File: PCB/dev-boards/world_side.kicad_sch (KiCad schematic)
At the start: 1 part, among them U1 NUCLEO-F429ZI

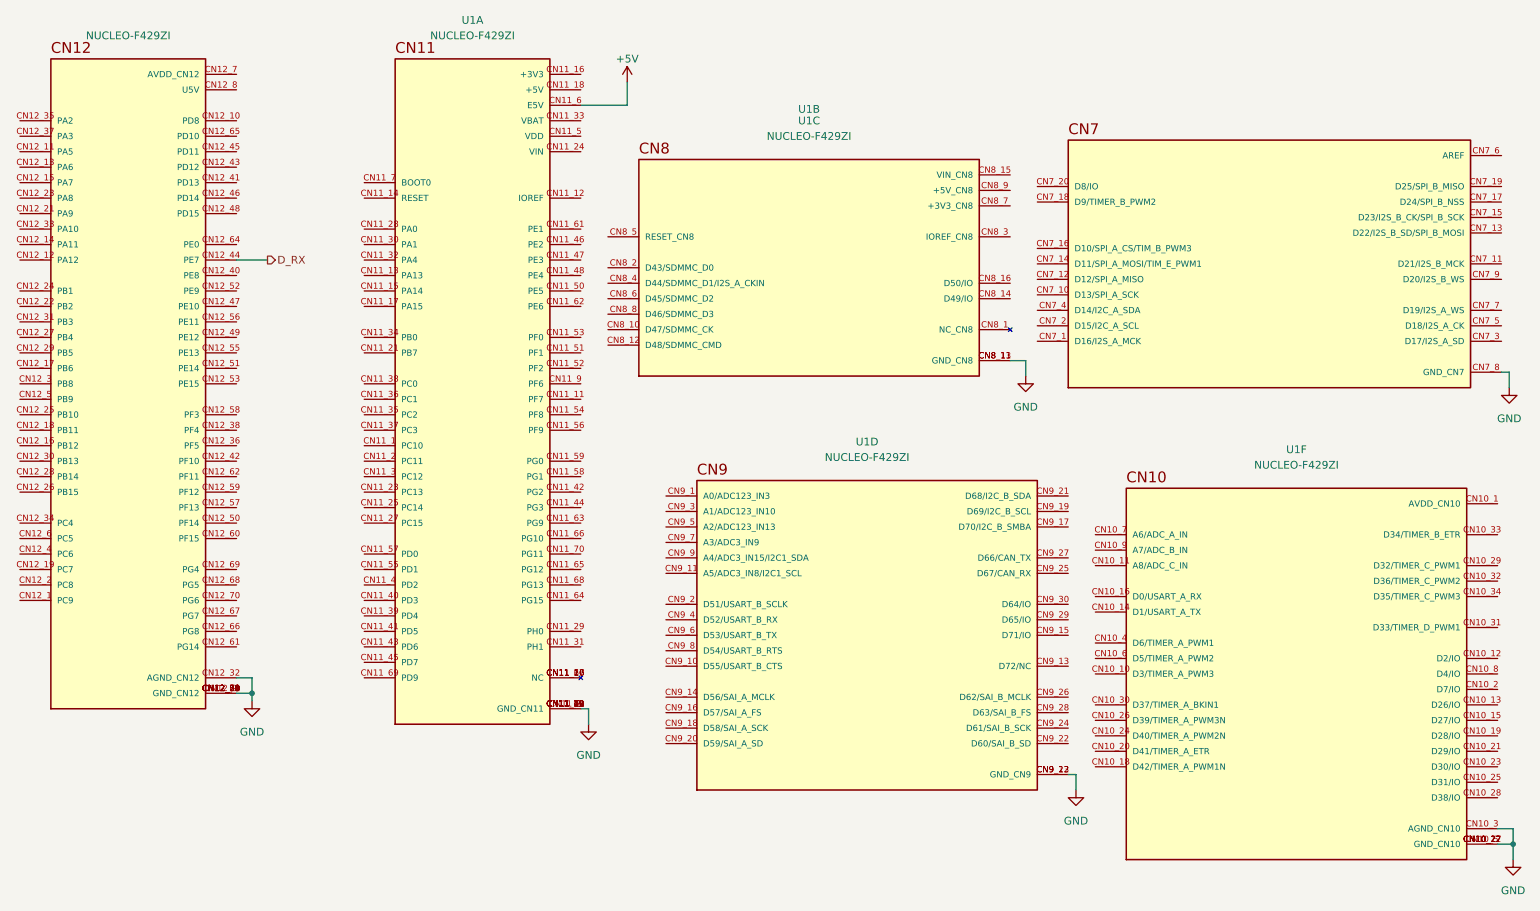
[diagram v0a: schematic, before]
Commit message: PCB board updates
Signed-off-by: Andrew Balmos <abalmos@purdue.edu>
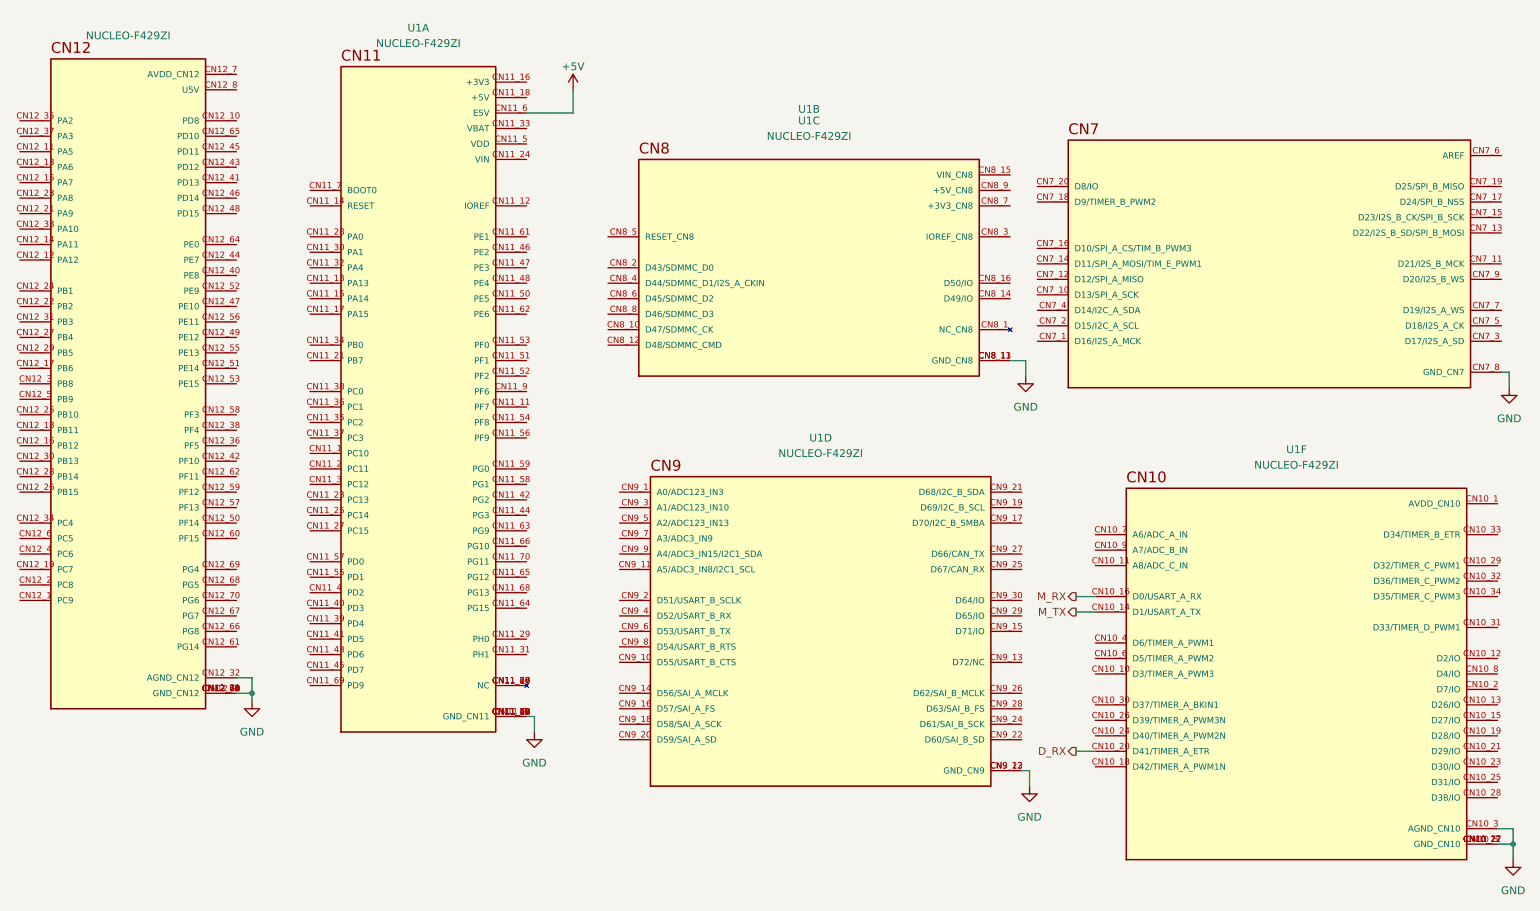
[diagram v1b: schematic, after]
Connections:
- net D_RX: now also U1.CN10_20 (D41/TIMER_A_ETR); no longer U1.CN12_44 (PE7)
- net M_TX: now reaches U1.CN10_14 (D1/USART_A_TX)
- net M_RX: now reaches U1.CN10_16 (D0/USART_A_RX)
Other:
- moved on the sheet: U1A, U1D
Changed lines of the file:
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@@
   (junction (at 55.245 128.27) (diameter 0) (color 0 0 0 0)
   )
-  (wire (pts (xy 116.84 27.94) (xy 116.84 31.75))
+  (wire (pts (xy 107.95 29.21) (xy 107.95 33.02))
     (stroke (width 0) (type default))
   )
@@
     (stroke (width 0) (type default))
   )
-  (wire (pts (xy 52.705 57.15) (xy 57.785 57.15))
-    (stroke (width 0) (type default))
-  )
   (wire (pts (xy 179.705 73.66) (xy 182.245 73.66))
     (stroke (width 0) (type default))
   )
-  (wire (pts (xy 190.5 141.605) (xy 190.5 144.145))
-    (stroke (width 0) (type default))
-  )
-  (wire (pts (xy 189.23 141.605) (xy 190.5 141.605))
+  (wire (pts (xy 182.88 140.97) (xy 182.88 143.51))
+    (stroke (width 0) (type default))
+  )
+  (wire (pts (xy 181.61 140.97) (xy 182.88 140.97))
     (stroke (width 0) (type default))
   )
@@
     (stroke (width 0) (type default))
   )
-  (wire (pts (xy 110.49 130.81) (xy 110.49 133.35))
+  (wire (pts (xy 101.6 132.08) (xy 101.6 134.62))
+    (stroke (width 0) (type default))
+  )
+  (wire (pts (xy 190.5 137.795) (xy 193.675 137.795))
     (stroke (width 0) (type default))
   )
@@
     (stroke (width 0) (type default))
   )
+  (wire (pts (xy 190.5 112.395) (xy 193.675 112.395))
+    (stroke (width 0) (type default))
+  )
+  (wire (pts (xy 190.5 114.935) (xy 193.675 114.935))
+    (stroke (width 0) (type default))
+  )
   (wire (pts (xy 259.715 150.495) (xy 262.255 150.495))
     (stroke (width 0) (type default))
@@
     (stroke (width 0) (type default))
   )
-  (wire (pts (xy 109.22 130.81) (xy 110.49 130.81))
+  (wire (pts (xy 100.33 132.08) (xy 101.6 132.08))
     (stroke (width 0) (type default))
   )
@@
     (stroke (width 0) (type default))
   )
-  (wire (pts (xy 109.22 31.75) (xy 116.84 31.75))
-    (stroke (width 0) (type default))
-  )
-  (hierarchical_label "D_RX" (shape output) (at 57.785 57.15 0) (fields_autoplaced)
-    (effects (font (size 1.27 1.27)) (justify left))
-  )
-  (symbol (lib_id "power:GND") (at 190.5 144.145 0) (unit 1)
+  (wire (pts (xy 100.33 33.02) (xy 107.95 33.02))
+    (stroke (width 0) (type default))
+  )
+  (hierarchical_label "M_TX" (shape output) (at 190.5 114.935 180) (fields_autoplaced)
+    (effects (font (size 1.27 1.27)) (justify right))
+  )
+  (hierarchical_label "D_RX" (shape output) (at 190.5 137.795 180) (fields_autoplaced)
+    (effects (font (size 1.27 1.27)) (justify right))
+  )
+  (hierarchical_label "M_RX" (shape output) (at 190.5 112.395 180) (fields_autoplaced)
+    (effects (font (size 1.27 1.27)) (justify right))
+  )
+  (symbol (lib_id "power:GND") (at 182.88 143.51 0) (unit 1)
     (in_bom yes) (on_board yes) (dnp no) (fields_autoplaced)
-    (property "Reference" "#PWR04" (at 190.5 150.495 0)
-      (effects (font (size 1.27 1.27)) hide)
-    )
-    (property "Value" "GND" (at 190.5 149.225 0)
+    (property "Reference" "#PWR04" (at 182.88 149.86 0)
+      (effects (font (size 1.27 1.27)) hide)
+    )
+    (property "Value" "GND" (at 182.88 148.59 0)
       (effects (font (size 1.27 1.27)))
     )
-    (property "Footprint" "" (at 190.5 144.145 0)
-      (effects (font (size 1.27 1.27)) hide)
-    )
-    (property "Datasheet" "" (at 190.5 144.145 0)
+    (property "Footprint" "" (at 182.88 143.51 0)
+      (effects (font (size 1.27 1.27)) hide)
+    )
+    (property "Datasheet" "" (at 182.88 143.51 0)
       (effects (font (size 1.27 1.27)) hide)
     )
@@
     )
   )
-  (symbol (lib_id "power:+5V") (at 116.84 27.94 0) (unit 1)
+  (symbol (lib_id "power:+5V") (at 107.95 29.21 0) (unit 1)
     (in_bom yes) (on_board yes) (dnp no) (fields_autoplaced)
-    (property "Reference" "#PWR016" (at 116.84 31.75 0)
-      (effects (font (size 1.27 1.27)) hide)
-    )
-    (property "Value" "+5V" (at 116.84 24.13 0)
+    (property "Reference" "#PWR016" (at 107.95 33.02 0)
+      (effects (font (size 1.27 1.27)) hide)
+    )
+    (property "Value" "+5V" (at 107.95 25.4 0)
       (effects (font (size 1.27 1.27)))
     )
-    (property "Footprint" "" (at 116.84 27.94 0)
-      (effects (font (size 1.27 1.27)) hide)
-    )
-    (property "Datasheet" "" (at 116.84 27.94 0)
+    (property "Footprint" "" (at 107.95 29.21 0)
+      (effects (font (size 1.27 1.27)) hide)
+    )
+    (property "Datasheet" "" (at 107.95 29.21 0)
       (effects (font (size 1.27 1.27)) hide)
     )
@@
     )
   )
-  (symbol (lib_id "Nucleo-144:NUCLEO-F429ZI") (at 156.21 118.745 0) (unit 4)
+  (symbol (lib_id "Nucleo-144:NUCLEO-F429ZI") (at 148.59 118.11 0) (unit 4)
     (in_bom yes) (on_board yes) (dnp no) (fields_autoplaced)
-    (property "Reference" "U1" (at 156.21 86.995 0)
+    (property "Reference" "U1" (at 148.59 86.36 0)
       (effects (font (size 1.27 1.27)))
     )
-    (property "Value" "NUCLEO-F429ZI" (at 156.21 89.535 0)
+    (property "Value" "NUCLEO-F429ZI" (at 148.59 88.9 0)
       (effects (font (size 1.27 1.27)))
     )
-    (property "Footprint" "MODULE_NUCLEO-F429ZI" (at 156.21 118.745 0)
-      (effects (font (size 1.27 1.27)) (justify bottom) hide)
-    )
-    (property "Datasheet" "" (at 156.21 118.745 0)
-      (effects (font (size 1.27 1.27)) hide)
-    )
-    (property "PARTREV" "8" (at 156.21 118.745 0)
-      (effects (font (size 1.27 1.27)) (justify bottom) hide)
-    )
-    (property "MANUFACTURER" "STMicroelectronics" (at 156.21 118.745 0)
-      (effects (font (size 1.27 1.27)) (justify bottom) hide)
-    )
-    (property "MAXIMUM_PACKAGE_HEIGHT" "N/A" (at 156.21 118.745 0)
-      (effects (font (size 1.27 1.27)) (justify bottom) hide)
-    )
-    (property "STANDARD" "Manufacturer Recommendations" (at 156.21 118.745 0)
+    (property "Footprint" "MODULE_NUCLEO-F429ZI" (at 148.59 118.11 0)
+      (effects (font (size 1.27 1.27)) (justify bottom) hide)
+    )
+    (property "Datasheet" "" (at 148.59 118.11 0)
+      (effects (font (size 1.27 1.27)) hide)
+    )
+    (property "PARTREV" "8" (at 148.59 118.11 0)
+      (effects (font (size 1.27 1.27)) (justify bottom) hide)
+    )
+    (property "MANUFACTURER" "STMicroelectronics" (at 148.59 118.11 0)
+      (effects (font (size 1.27 1.27)) (justify bottom) hide)
+    )
+    (property "MAXIMUM_PACKAGE_HEIGHT" "N/A" (at 148.59 118.11 0)
+      (effects (font (size 1.27 1.27)) (justify bottom) hide)
+    )
+    (property "STANDARD" "Manufacturer Recommendations" (at 148.59 118.11 0)
       (effects (font (size 1.27 1.27)) (justify bottom) hide)
     )
@@
     )
   )
-  (symbol (lib_id "power:GND") (at 110.49 133.35 0) (unit 1)
+  (symbol (lib_id "power:GND") (at 101.6 134.62 0) (unit 1)
     (in_bom yes) (on_board yes) (dnp no) (fields_autoplaced)
-    (property "Reference" "#PWR015" (at 110.49 139.7 0)
-      (effects (font (size 1.27 1.27)) hide)
-    )
-    (property "Value" "GND" (at 110.49 138.43 0)
+    (property "Reference" "#PWR015" (at 101.6 140.97 0)
+      (effects (font (size 1.27 1.27)) hide)
+    )
+    (property "Value" "GND" (at 101.6 139.7 0)
       (effects (font (size 1.27 1.27)))
     )
-    (property "Footprint" "" (at 110.49 133.35 0)
-      (effects (font (size 1.27 1.27)) hide)
-    )
-    (property "Datasheet" "" (at 110.49 133.35 0)
+    (property "Footprint" "" (at 101.6 134.62 0)
+      (effects (font (size 1.27 1.27)) hide)
+    )
+    (property "Datasheet" "" (at 101.6 134.62 0)
       (effects (font (size 1.27 1.27)) hide)
     )
@@
     )
   )
-  (symbol (lib_id "Nucleo-144:NUCLEO-F429ZI") (at 91.44 77.47 0) (unit 1)
+  (symbol (lib_id "Nucleo-144:NUCLEO-F429ZI") (at 82.55 78.74 0) (unit 1)
     (in_bom yes) (on_board yes) (dnp no) (fields_autoplaced)
-    (property "Reference" "U1" (at 91.44 17.78 0)
+    (property "Reference" "U1" (at 82.55 19.05 0)
       (effects (font (size 1.27 1.27)))
     )
-    (property "Value" "NUCLEO-F429ZI" (at 91.44 20.32 0)
+    (property "Value" "NUCLEO-F429ZI" (at 82.55 21.59 0)
       (effects (font (size 1.27 1.27)))
     )
-    (property "Footprint" "MODULE_NUCLEO-F429ZI" (at 91.44 77.47 0)
-      (effects (font (size 1.27 1.27)) (justify bottom) hide)
-    )
-    (property "Datasheet" "" (at 91.44 77.47 0)
-      (effects (font (size 1.27 1.27)) hide)
-    )
-    (property "PARTREV" "8" (at 91.44 77.47 0)
-      (effects (font (size 1.27 1.27)) (justify bottom) hide)
-    )
-    (property "MANUFACTURER" "STMicroelectronics" (at 91.44 77.47 0)
-      (effects (font (size 1.27 1.27)) (justify bottom) hide)
-    )
-    (property "MAXIMUM_PACKAGE_HEIGHT" "N/A" (at 91.44 77.47 0)
-      (effects (font (size 1.27 1.27)) (justify bottom) hide)
-    )
-    (property "STANDARD" "Manufacturer Recommendations" (at 91.44 77.47 0)
-      (effects (font (size 1.27 1.27)) (justify bottom) hide)
-    )
+    (property "Footprint" "MODULE_NUCLEO-F429ZI" (at 82.55 78.74 0)
+      (effects (font (size 1.27 1.27)) (justify bottom) hide)
+    )
+    (property "Datasheet" "" (at 82.55 78.74 0)
+      (effects (font (size 1.27 1.27)) hide)
+    )
+    (property "PARTREV" "8" (at 82.55 78.74 0)
+      (effects (font (size 1.27 1.27)) (justify bottom) hide)
+    )
+    (property "MANUFACTURER" "STMicroelectronics" (at 82.55 78.74 0)
+      (effects (font (size 1.27 1.27)) (justify bottom) hide)
+    )
+    (property "MAXIMUM_PACKAGE_HEIGHT" "N/A" (at 82.55 78.74 0)
+      (effects (font (size 1.27 1.27)) (justify bottom) hide)
+    )
+    (property "STANDARD" "Manufacturer Recommendations" (at 82.55 78.74 0)
+      (effects (font (size 1.27 1.27)) (justify bottom) hide)
+    )
